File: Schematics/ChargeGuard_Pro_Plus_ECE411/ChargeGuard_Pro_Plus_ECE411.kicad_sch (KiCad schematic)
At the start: 19 parts, among them J1 Barrel_Jack_MountingPin, J2 Screw_Terminal_01x02, J3 Screw_Terminal_01x02, J4 Screw_Terminal_01x02, J5 Screw_Terminal_01x02, J6 Screw_Terminal_01x02, J7 Screw_Terminal_01x02, K1 SANYOU_SRD_Form_C, Q1 2N3906, Q3 2N7000

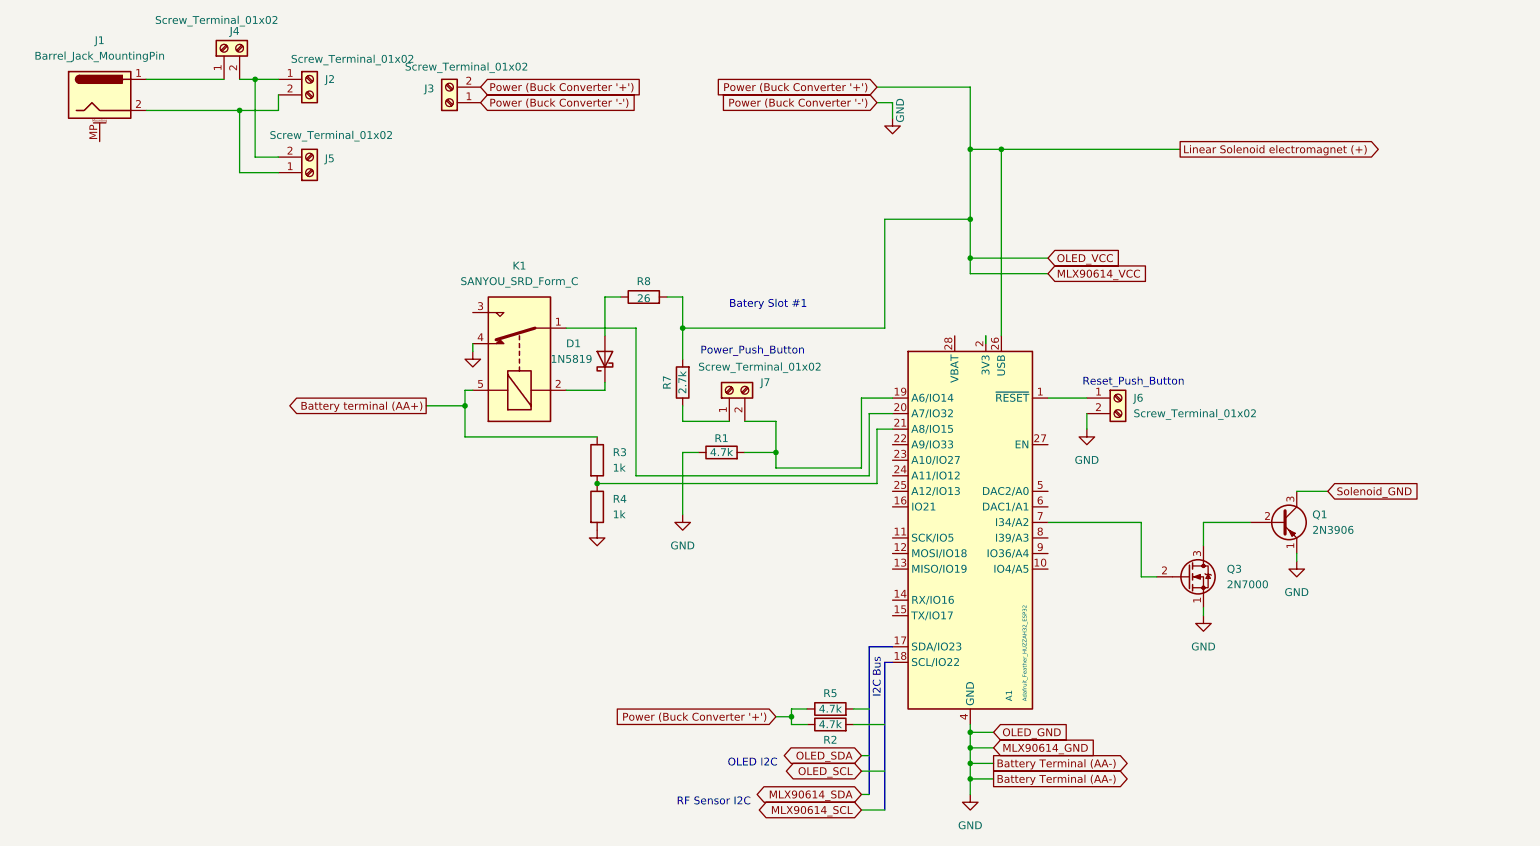
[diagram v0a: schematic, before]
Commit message: Add files via upload
Updated Version of Schematic as well as PCB Design
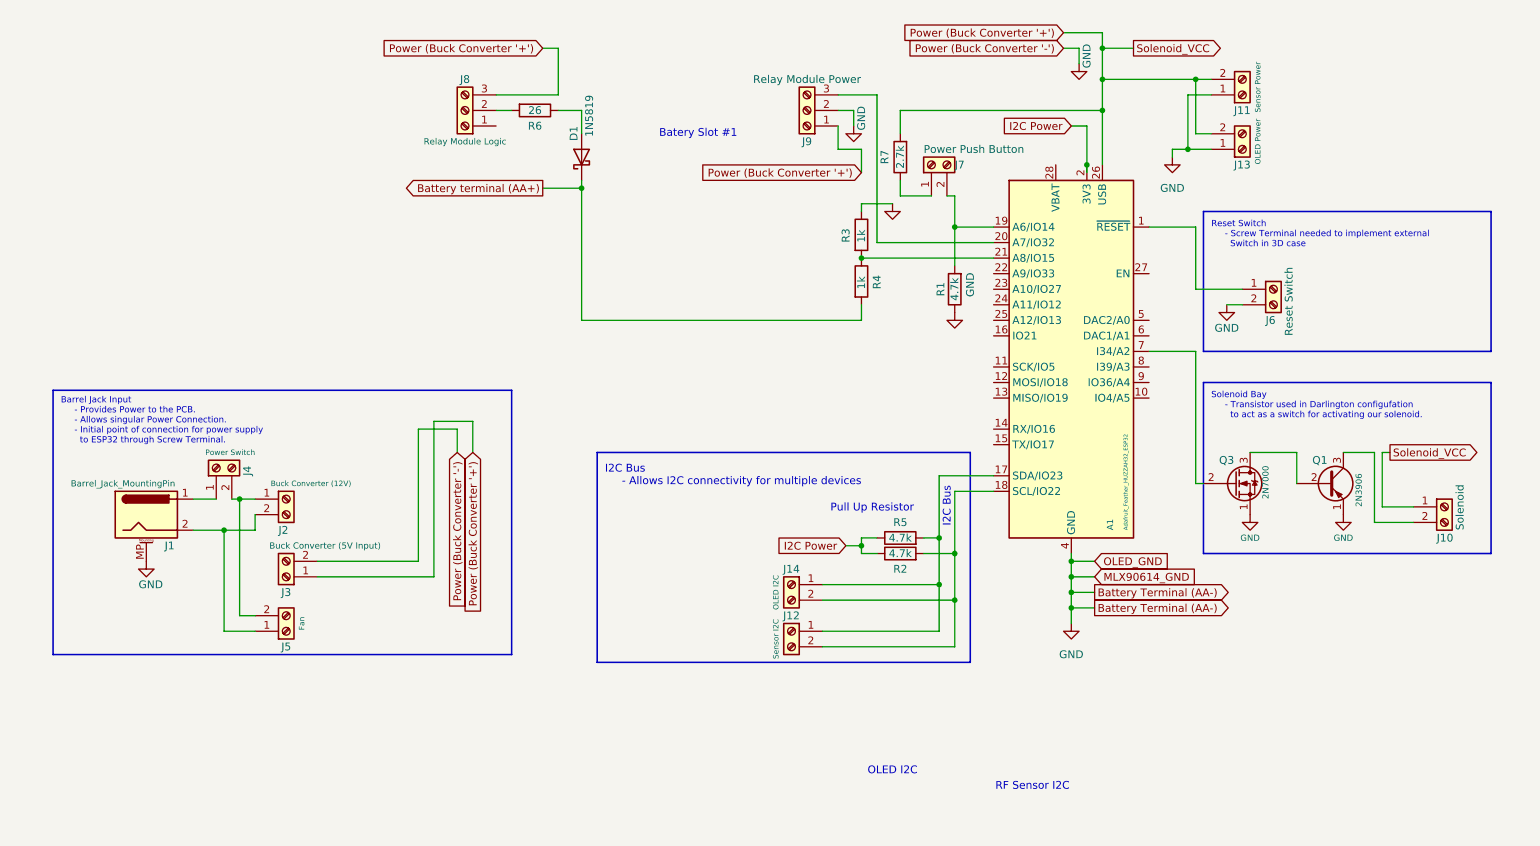
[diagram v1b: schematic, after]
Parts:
- removed K1: SANYOU_SRD_Form_C, Relay_THT:Relay_SPDT_SANYOU_SRD_Series_Form_C, symbol Relay:SANYOU_SRD_Form_C
- removed R8: 26, Resistor_THT:R_Axial_DIN0204_L3.6mm_D1.6mm_P5.08mm_Horizontal, symbol Device:R
- added J10: Solenoid, TerminalBlock_MetzConnect:TerminalBlock_MetzConnect_Type101_RT01602HBWC_1x02_P5.08mm_Horizontal, symbol Connector:Screw_Terminal_01x02
- added J11: Sensor Power, TerminalBlock_MetzConnect:TerminalBlock_MetzConnect_Type101_RT01602HBWC_1x02_P5.08mm_Horizontal, symbol Connector:Screw_Terminal_01x02
- added J12: Sensor I2C, TerminalBlock_MetzConnect:TerminalBlock_MetzConnect_Type101_RT01602HBWC_1x02_P5.08mm_Horizontal, symbol Connector:Screw_Terminal_01x02
- added J13: OLED Power, TerminalBlock_MetzConnect:TerminalBlock_MetzConnect_Type101_RT01602HBWC_1x02_P5.08mm_Horizontal, symbol Connector:Screw_Terminal_01x02
- added J14: OLED I2C, TerminalBlock_MetzConnect:TerminalBlock_MetzConnect_Type101_RT01602HBWC_1x02_P5.08mm_Horizontal, symbol Connector:Screw_Terminal_01x02
- added J8: Relay Module Logic, TerminalBlock_MetzConnect:TerminalBlock_MetzConnect_Type055_RT01503HDWU_1x03_P5.00mm_Horizontal, symbol Connector:Screw_Terminal_01x03
- added J9: Relay Module Power, TerminalBlock_MetzConnect:TerminalBlock_MetzConnect_Type055_RT01503HDWU_1x03_P5.00mm_Horizontal, symbol Connector:Screw_Terminal_01x03
- added R6: 26, Resistor_THT:R_Axial_DIN0204_L3.6mm_D1.6mm_P5.08mm_Horizontal, symbol Device:R
- J2: value Screw_Terminal_01x02 -> Buck Converter (12V); footprint TerminalBlock_MetzConnect:TerminalBlock_MetzConnect_360291_1x01_Horizontal_ScrewM3.0_Boxed -> TerminalBlock_MetzConnect:TerminalBlock_MetzConnect_Type101_RT01602HBWC_1x02_P5.08mm_Horizontal
- J3: value Screw_Terminal_01x02 -> Buck Converter (5V Input); footprint TerminalBlock_MetzConnect:TerminalBlock_MetzConnect_360291_1x01_Horizontal_ScrewM3.0_Boxed -> TerminalBlock_MetzConnect:TerminalBlock_MetzConnect_Type101_RT01602HBWC_1x02_P5.08mm_Horizontal
- J4: value Screw_Terminal_01x02 -> Power Switch; footprint TerminalBlock_MetzConnect:TerminalBlock_MetzConnect_360291_1x01_Horizontal_ScrewM3.0_Boxed -> TerminalBlock_MetzConnect:TerminalBlock_MetzConnect_Type101_RT01602HBWC_1x02_P5.08mm_Horizontal
- J5: value Screw_Terminal_01x02 -> Fan; footprint TerminalBlock_MetzConnect:TerminalBlock_MetzConnect_360291_1x01_Horizontal_ScrewM3.0_Boxed -> TerminalBlock_MetzConnect:TerminalBlock_MetzConnect_Type101_RT01602HBWC_1x02_P5.08mm_Horizontal
- J6: value Screw_Terminal_01x02 -> Reset Switch; footprint TerminalBlock_MetzConnect:TerminalBlock_MetzConnect_360291_1x01_Horizontal_ScrewM3.0_Boxed -> TerminalBlock_MetzConnect:TerminalBlock_MetzConnect_Type101_RT01602HBWC_1x02_P5.08mm_Horizontal
- J7: value Screw_Terminal_01x02 -> Power Push Button; footprint TerminalBlock_MetzConnect:TerminalBlock_MetzConnect_360291_1x01_Horizontal_ScrewM3.0_Boxed -> TerminalBlock_MetzConnect:TerminalBlock_MetzConnect_Type101_RT01602HBWC_1x02_P5.08mm_Horizontal
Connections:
- net Battery terminal (AA+): now also D1.1 (K), R4.2; no longer R3.1
- net GND: now also J1.MP (MountPin), J3.2 (Pin_2), R3.1, J11.1 (Pin_1), J13.1 (Pin_1), J9.2 (Pin_2); no longer J3.1 (Pin_1), R4.2
- net at D1.2 (A): now also R6.1
- net at A1.17 (SDA/IO23): now also R5.2, J12.1 (Pin_1), J14.1 (Pin_1)
- net at A1.18 (SCL/IO22): now also R2.2, J12.2 (Pin_2), J14.2 (Pin_2)
- net I2C Power: now reaches A1.2 (3V3)
- net I2C Power: now also R2.1, R5.1
- net at A1.20 (A7/IO32): now also J9.3 (Pin_3)
- removed net Linear Solenoid electromagnet (+): A1.26 (USB), J3.2 (Pin_2), R2.1, R5.1, R7.2
- net Solenoid_GND: no longer names the net of Q1.3 (C)
- net Solenoid_GND: now also J10.2 (Pin_2)
- new net: J8.2 (Pin_2), R6.2
- new net Power (Buck Converter '+'): A1.26 (USB), J10.1 (Pin_1), J11.2 (Pin_2), J13.2 (Pin_2), J3.1 (Pin_1), J8.3 (Pin_3), J9.1 (Pin_1), R7.2
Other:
- note added: "Barrel Jack Input - Provides Power to the PCB. - Allows singular Power Connection. - Initial point of connection for power supply to ESP32 through Screw Terminal."
- note added: "I2C Bus - Allows I2C connectivity for multiple devices"
- note added: "Pull Up Resistor"
- note added: "Reset Switch - Screw Terminal needed to implement external Switch in 3D case"
- note added: "Solenoid Bay - Transistor used in Darlington configufation to act as a switch for activating our solenoid."
- note removed: "Power_Push_Button"
- note removed: "Reset_Push_Button"
- moved on the sheet: A1, J1, J2, J3, J4, J5, J6, J7, Q1, Q3, R1, R2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
